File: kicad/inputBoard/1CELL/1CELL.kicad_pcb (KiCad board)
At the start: 2 copper layers, 5 parts, among them J1 Conn_01x02_Pin, Q1 Q_NMOS_GSD, Q2 Q_NMOS_GSD, SW1 SW_Push, SW2 SW_Push

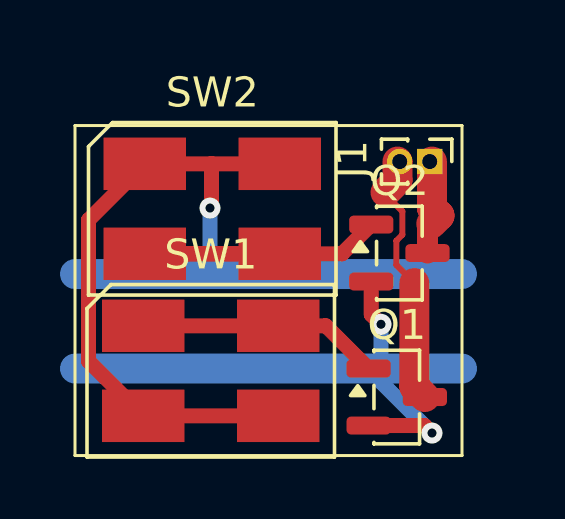
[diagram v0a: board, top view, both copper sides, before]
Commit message: finish main input board
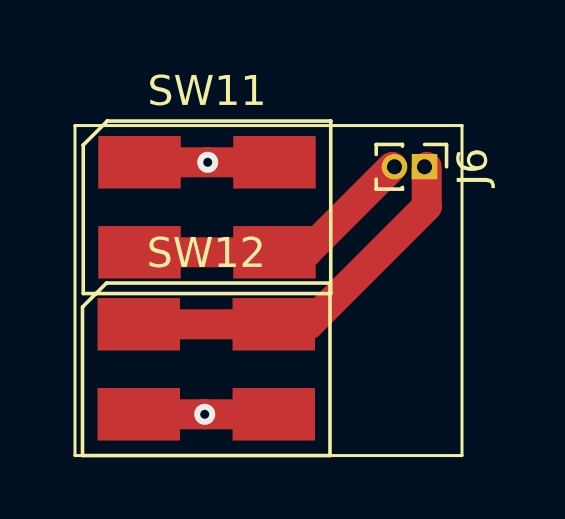
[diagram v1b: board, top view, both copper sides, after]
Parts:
- removed J1: Conn_01x02_Pin, Connector_PinHeader_1.00mm:PinHeader_1x02_P1.00mm_Vertical
- removed Q1, Q2: Q_NMOS_GSD, Package_TO_SOT_SMD:SOT-23
- removed SW1, SW2: SW_Push, Button_Switch_SMD:SW_4.5mm
- added J6: Conn_01x02_Pin, Connector_PinHeader_1.00mm:PinHeader_1x02_P1.00mm_Vertical, F.Cu at (129.0, 76.3)
- added SW11: SW_Push, Button_Switch_SMD:SW_4.5mm, F.Cu at (121.8, 77.7)
- added SW12: SW_Push, Button_Switch_SMD:SW_4.5mm, F.Cu at (121.7, 83.1)
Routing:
- net +5V: track 35.5 -> 0.00 mm, vias 1 -> 0
- net Net-(J6-Pin_1): track 0.00 -> 12.6 mm
- net Net-(Q2-G): track 12.5 -> 0.00 mm
- net GND: track 21.0 -> 9.00 mm
- net Net-(J6-Pin_2): track 0.00 -> 9.61 mm
- net Net-(J1-Pin_2): track 8.73 -> 0.00 mm
- net Net-(Q1-G): track 8.10 -> 0.00 mm
- net Net-(J1-Pin_1): track 3.32 -> 0.00 mm
